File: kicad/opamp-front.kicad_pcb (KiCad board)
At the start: 2 copper layers, 87 parts, among them J1 B+, J2 SPK, J3 INPUT, J4 GND, J5 B-, J6 GND, Q1 2N5551, Q10 2N2906, Q11 MJL3281C, Q12 2N2904, Q13 MJL1302C, Q2 BD139, Q3 BD140, Q4 BD139, Q5 BD139, Q6 2N5401, Q7 2N5551, Q8 2N5401, Q9 BD140, U1 LM4562

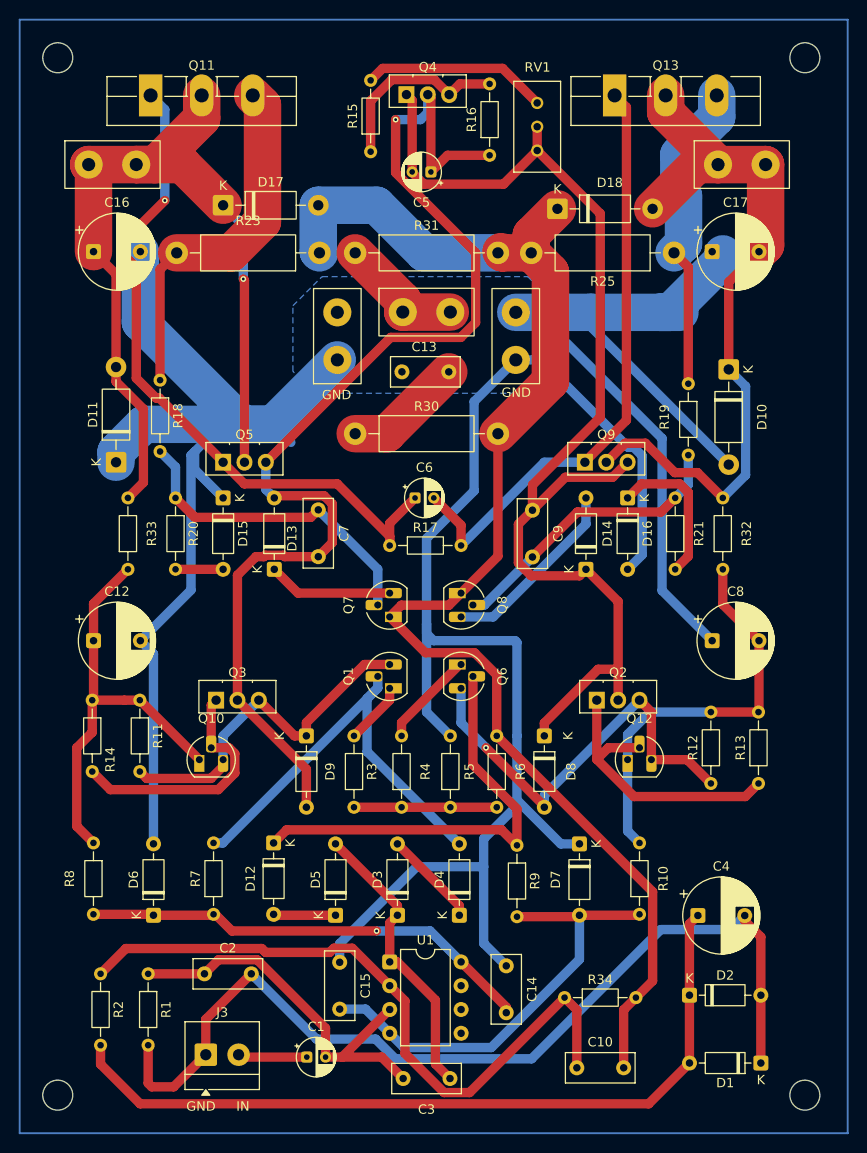
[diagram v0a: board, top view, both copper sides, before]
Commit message: WIP
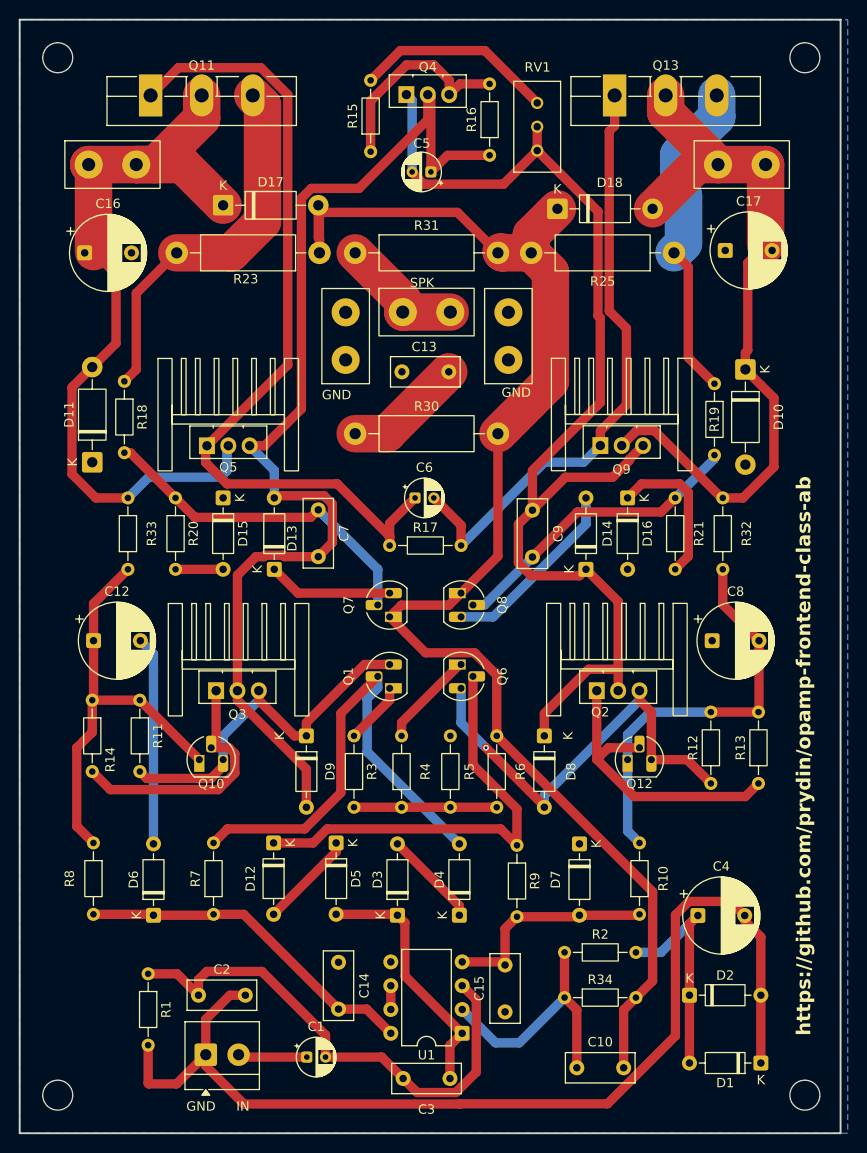
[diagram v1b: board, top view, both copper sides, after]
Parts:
- added REF**: Heatsink, Custom:Heatsink, F.Cu at (79.7, 75.2)
- added REF**: Heatsink, Custom:Heatsink, F.Cu at (121.2, 101.3)
- added REF**: Heatsink, Custom:Heatsink, F.Cu at (80.8, 101.4)
- added REF**: Heatsink, Custom:Heatsink, F.Cu at (121.7, 75.2)
- R18, R19: value 1k -> 100
- R20, R21: value 4.7k -> 1.5k
- moved R2 49.6 mm to (115.6, 133.6), turned to 0 degrees
- moved C15 18.4 mm to (109.2, 140.0), turned to 90 degrees
- moved C14 17.9 mm to (91.4, 134.7)
- moved U1 10.9 mm to (104.6, 142.2), turned to 180 degrees
- moved D5 7.72 mm to (91.2, 121.9), turned to -90 degrees
- moved R18 3.81 mm to (68.6, 72.6)
- moved R19 2.79 mm to (131.6, 72.9)
- moved D11 2.54 mm to (65.2, 81.3)
- moved Q5 2.47 mm to (77.4, 79.5)
- moved Q9 2.43 mm to (119.4, 79.5)
- moved C2 2.37 mm to (76.5, 138.2)
- moved D10 1.78 mm to (134.9, 71.4)
- moved C17 1.40 mm to (132.7, 58.7)
- moved Q2 1.02 mm to (119.0, 105.7)
- moved Q3 1.02 mm to (78.4, 105.7)
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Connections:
- U1 pad 5: (no net) -> GND
- U1 pad 6: (no net) -> Net-(U1B--)
- U1 pad 7: (no net) -> Net-(U1B--)
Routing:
- net GND: track 358.7 -> 22.3 mm
- net Net-(D1-A): track 84.6 -> 24.4 mm
- net Net-(U1A--): track 72.9 -> 27.3 mm
- net -15V: track 49.1 -> 23.2 mm
- net Net-(Q11-B): track 74.2 -> 90.1 mm, vias 1 -> 0
- net Net-(U1A-+): track 42.1 -> 55.5 mm
- net GNDA: track 101.7 -> 114.6 mm
- net +15V: track 48.8 -> 37.2 mm, vias 1 -> 0
- net /B+: track 94.7 -> 85.2 mm, vias 1 -> 0
- net Net-(D13-A): track 129.3 -> 121.6 mm, vias 1 -> 0
- net Net-(D4-A): track 46.8 -> 52.3 mm
- net Net-(D17-A): track 149.5 -> 154.4 mm
- net Net-(D3-K): track 31.3 -> 27.3 mm
- net Net-(D12-A): track 6.65 -> 10.4 mm
- net Net-(U1B--): track 0.00 -> 2.54 mm
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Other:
- board outline added: 87.6 x 118.9 mm
- board text added: "SPK"
- board text added: "https://github.com/prydin/opamp-frontend-class-ab"
